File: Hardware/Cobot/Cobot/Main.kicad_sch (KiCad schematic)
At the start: 22 parts, among them J1 USB_B_Micro, J2 Conn_02x02_Counter_Clockwise, U1 STM32L433RCTxP, U2 USBLC6-2SC6, U3 RFM95W-868S2

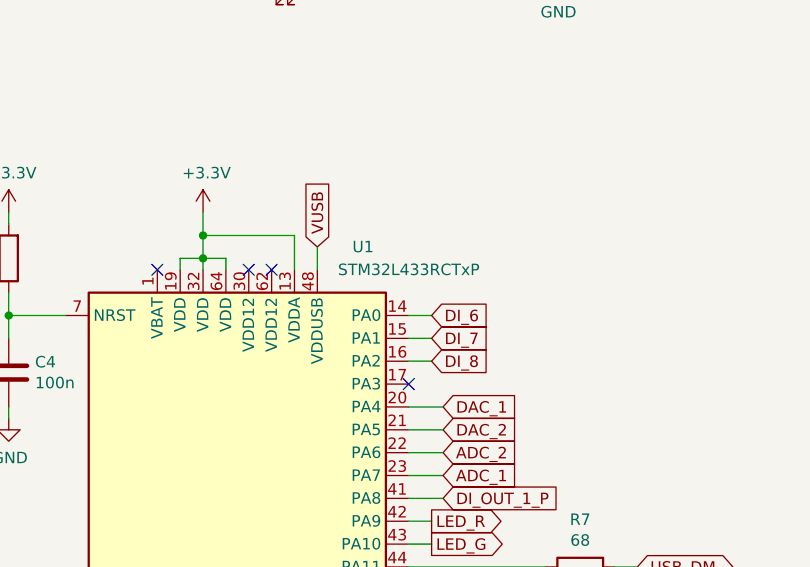
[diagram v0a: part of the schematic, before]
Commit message: Update Firmware
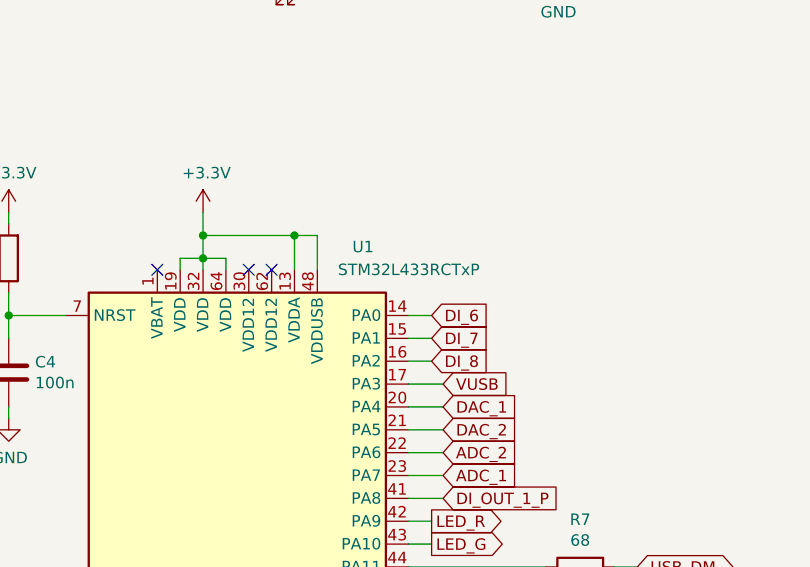
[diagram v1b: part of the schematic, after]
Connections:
- net +3.3V: now also U1.48 (VDDUSB)
- net VUSB: now also U1.17 (PA3); no longer U1.48 (VDDUSB)
- no-connect marks 11 -> 10
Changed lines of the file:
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@@
   (junction (at 67.31 73.66) (diameter 0) (color 0 0 0 0)
+  )
+  (junction (at 77.47 73.66) (diameter 0) (color 0 0 0 0)
   )
   (junction (at 27.94 45.72) (diameter 0) (color 0 0 0 0)
@@
   (no_connect (at 180.34 130.81))
   (no_connect (at 90.17 120.65))
-  (no_connect (at 90.17 90.17))
   (no_connect (at 62.23 77.47))
   (no_connect (at 52.07 118.11))
@@
     (stroke (width 0) (type default) (color 0 0 0 0))
   )
+  (wire (pts (xy 77.47 73.66) (xy 80.01 73.66))
+    (stroke (width 0) (type default) (color 0 0 0 0))
+  )
   (wire (pts (xy 106.68 38.1) (xy 110.49 38.1))
     (stroke (width 0) (type default) (color 0 0 0 0))
@@
     (stroke (width 0) (type default) (color 0 0 0 0))
   )
+  (wire (pts (xy 90.17 90.17) (xy 93.98 90.17))
+    (stroke (width 0) (type default) (color 0 0 0 0))
+  )
   (wire (pts (xy 49.53 138.43) (xy 52.07 138.43))
     (stroke (width 0) (type default) (color 0 0 0 0))
@@
     (stroke (width 0) (type default) (color 0 0 0 0))
   )
-  (wire (pts (xy 80.01 77.47) (xy 80.01 74.93))
+  (wire (pts (xy 80.01 73.66) (xy 80.01 77.47))
     (stroke (width 0) (type default) (color 0 0 0 0))
   )
@@
     )
   )
+  (global_label "VUSB" (shape input) (at 93.98 90.17 0) (fields_autoplaced)
+    (effects (font (size 1.27 1.27)) (justify left))
+    (property "Intersheet References" "${INTERSHEET_REFS}" (id 0) (at 101.2917 90.0906 0)
+      (effects (font (size 1.27 1.27)) (justify left) hide)
+    )
+  )
   (global_label "ADC_2" (shape input) (at 93.98 97.79 0) (fields_autoplaced)
     (effects (font (size 1.27 1.27)) (justify left))
@@
     )
   )
-  (global_label "VUSB" (shape input) (at 80.01 74.93 90) (fields_autoplaced)
-    (effects (font (size 1.27 1.27)) (justify left))
-    (property "Intersheet References" "${INTERSHEET_REFS}" (id 0) (at 6.35 26.67 0)
-      (effects (font (size 1.27 1.27)) hide)
-    )
-  )

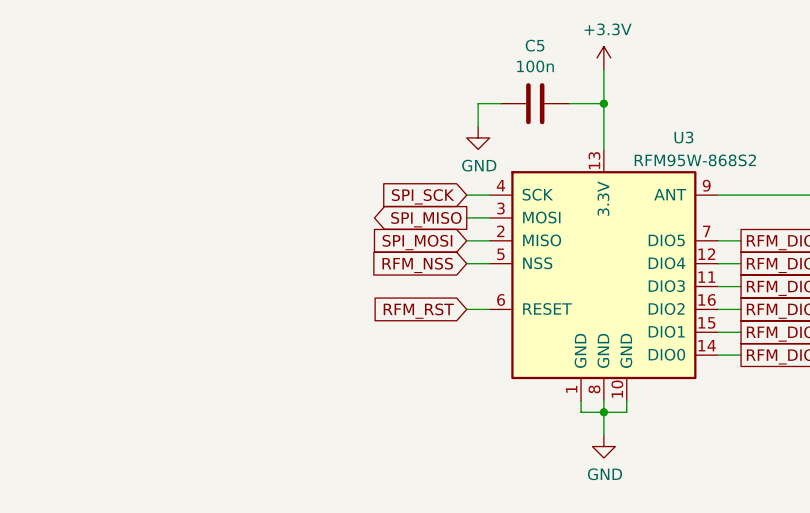
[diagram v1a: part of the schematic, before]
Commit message: Update HW and SW
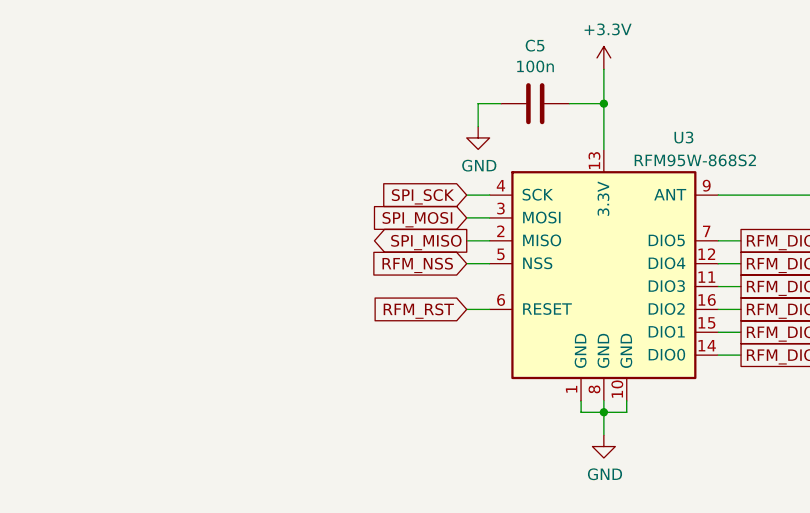
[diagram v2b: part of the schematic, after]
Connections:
- net SPI_MISO: now also U3.2 (MISO); no longer U3.3 (MOSI)
- net SPI_MOSI: now also U3.3 (MOSI); no longer U3.2 (MISO)
